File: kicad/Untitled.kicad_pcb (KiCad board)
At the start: 2 copper layers, 72.4 x 62.5 mm, 10 parts, among them J6 171825-6, U1 esp32_38_pins-custom_library, m1 2-171825-3, m2 2-171825-3, m3 2-171825-3, m4 2-171825-3

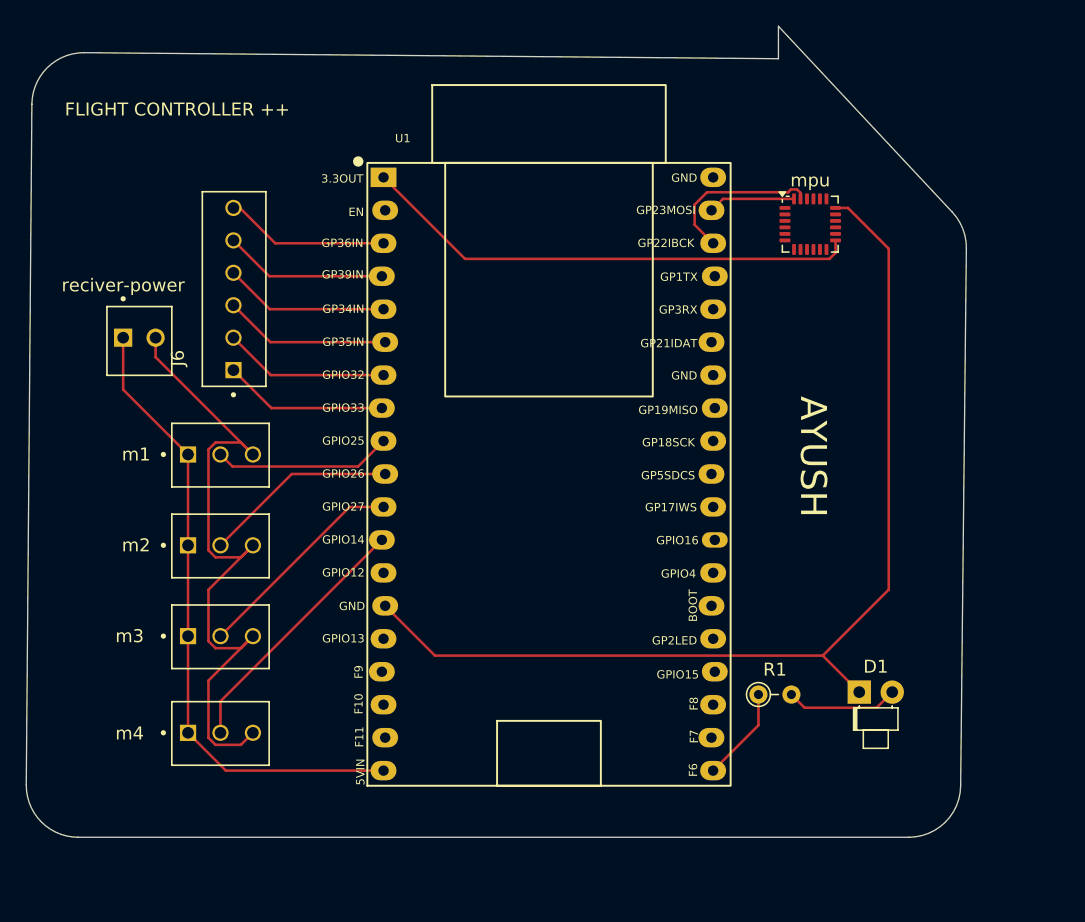
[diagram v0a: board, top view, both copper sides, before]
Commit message: updated pcb
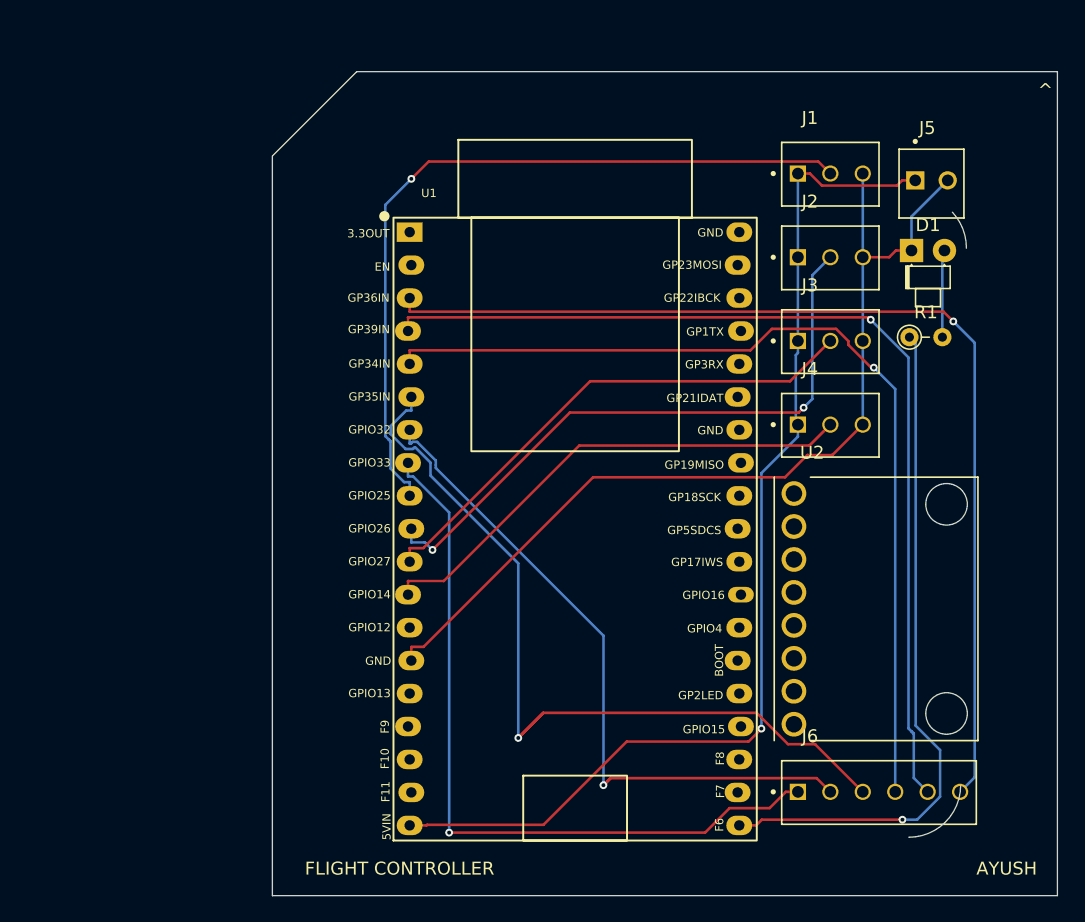
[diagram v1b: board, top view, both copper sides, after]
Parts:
- removed m1, m2, m3, m4: 2-171825-3, 2-171825-3 (1):TE_2-171825-3
- removed mpu: MPU-6050, Sensor_Motion:InvenSense_QFN-24_4x4mm_P0.5mm
- removed reciver-power: 171825-2, 171825-2:TE_171825-2
- added J1: 2-171825-3, 2-171825-3 (1):TE_2-171825-3, F.Cu at (176.0, 67.3)
- added J2: 2-171825-3, 2-171825-3 (1):TE_2-171825-3, F.Cu at (176.0, 73.8)
- added J3: 2-171825-3, 2-171825-3 (1):TE_2-171825-3, F.Cu at (176.0, 80.2)
- added J4: 2-171825-3, 2-171825-3 (1):TE_2-171825-3, F.Cu at (176.0, 86.7)
- added J5: 171825-2, 171825-2:TE_171825-2, F.Cu at (186.3, 67.9)
- added U2: MPU-6050, GY-521:MODULE_GY-521, F.Cu at (182.0, 100.9)
- moved J6 54.3 mm to (176.0, 115.0), turned to 0 degrees
- moved D1 34.3 mm to (184.8, 73.3)
- moved R1 29.9 mm to (184.6, 80.0)
- moved U1 4.68 mm to (146.1, 71.9)
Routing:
- net Net-(U1-GPI36): track 12.7 -> 80.7 mm, vias 0 -> 1
- net Net-(U1-GPI39): track 12.6 -> 75.2 mm, vias 0 -> 1
- net Net-(U1-GPI35): track 12.9 -> 72.7 mm, vias 0 -> 1
- net Net-(U1-GPI34): track 12.7 -> 72.3 mm, vias 0 -> 1
- net gnd: track 132.2 -> 72.8 mm
- net Net-(U1-GPIO25): track 13.8 -> 59.7 mm, vias 0 -> 1
- net Net-(U1-GPIO33): track 12.6 -> 58.2 mm, vias 0 -> 1
- net Net-(U1-GPIO6): track 7.31 -> 52.8 mm, vias 0 -> 1
- net Net-(U1-GPIO32): track 12.8 -> 55.3 mm, vias 0 -> 1
- net Net-(U1-3.3V): track 38.6 -> 0.00 mm
- net Net-(U1-5V): track 48.8 -> 83.9 mm, vias 0 -> 1
- net Net-(U1-GPIO26): track 15.0 -> 48.5 mm, vias 0 -> 2
- net Net-(U1-GPIO27): track 16.7 -> 40.1 mm
- net Net-(U1-GPIO14): track 20.0 -> 38.6 mm
- net Net-(U1-GPIO22): track 12.8 -> 0.00 mm
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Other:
- board size 72.4 x 62.5 mm -> 60.5 x 63.5 mm
- board text added: "FLIGHT CONTROLLER"
- board text added: "^"
- board text removed: "FLIGHT CONTROLLER ++"
